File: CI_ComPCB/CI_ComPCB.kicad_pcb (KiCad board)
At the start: 2 copper layers, 121.9 x 86.4 mm, 73 parts, among them IC301 TPS63020DSJR, IC401 TPS54331DR, J101 Conn_01x01_Male, J301 Connector_Conn_01x01_Male, J302 Connector_Conn_01x01_Male, J303 Connector_Conn_01x01_Male, J401 Connector_Conn_01x01_Male, J402 Conn_01x02_Male, J403 Conn_01x01_Male, J501 RJ45_LED_Shielded, J502 RJ45_LED_Shielded, J601 Conn_01x02_Male, J602 Conn_01x02_Male, J603 Conn_01x03_Male, J604 Conn_01x03_Male, J605 Conn_01x02_Male, K601 SRD-05VDC-SL-C, K602 SRD-05VDC-SL-C, Q201 Transistor_FET_IRF9540N, Q601 2N3904, Q602 2N3904, U101 ESP32s

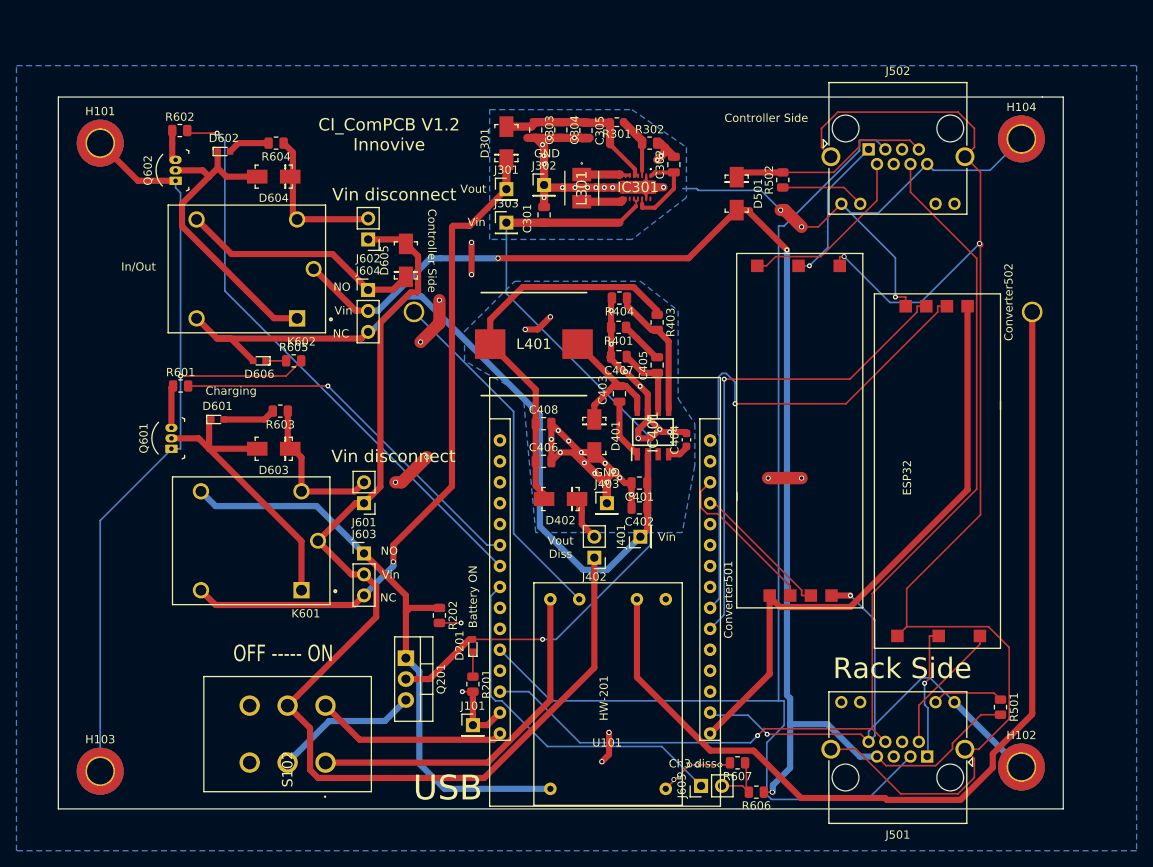
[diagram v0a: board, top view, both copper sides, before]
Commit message: Production1
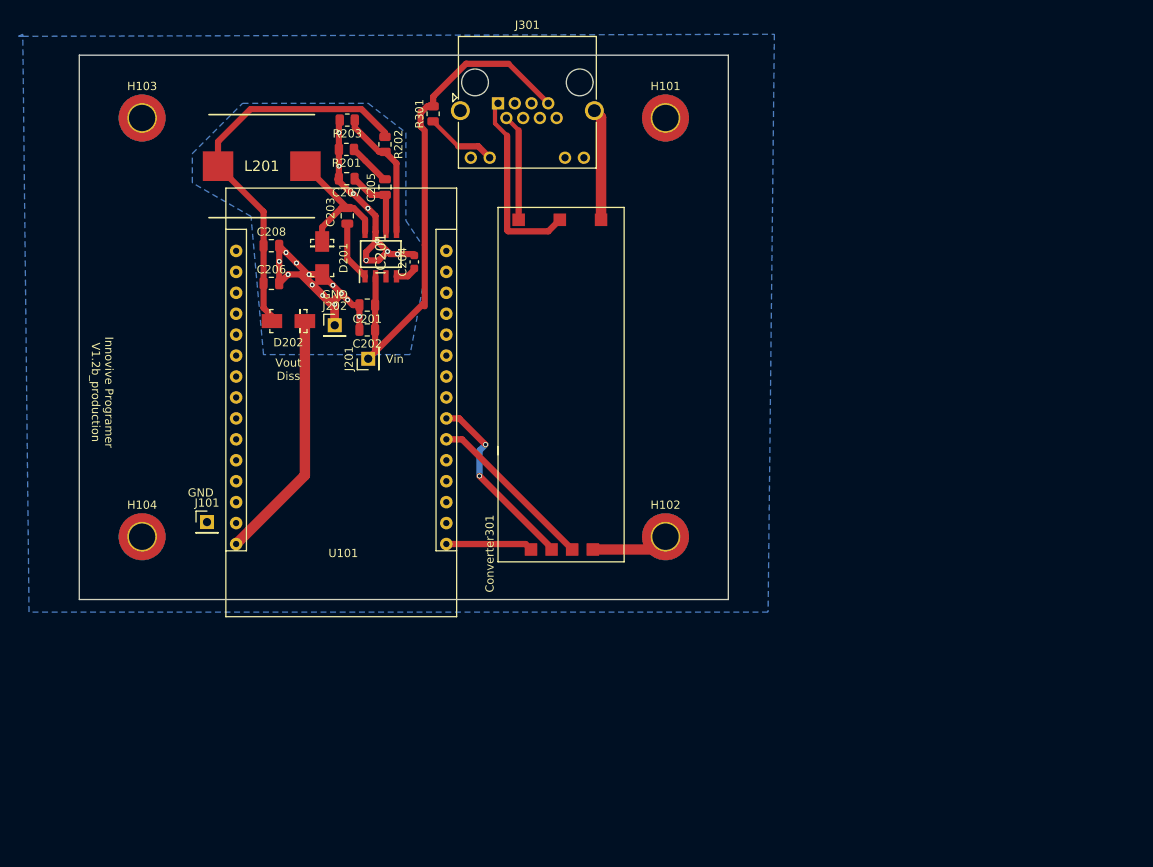
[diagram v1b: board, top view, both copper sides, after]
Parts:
- removed C301: 22uF, Capacitor_SMD:C_0805_2012Metric
- removed C302: 100nF, Capacitor_SMD:C_0805_2012Metric
- removed C303, C304, C305: 10uf, Capacitor_SMD:C_0805_2012Metric
- removed Converter501, Converter502: TxRx-RS485, CI_ComPCB:TXRX-AB
- removed the D201 at (145.8, 138.1)
- removed D301, D501, D605: SS34, digikey-footprints:DO-214AC
- removed D601, D602, D606: LTST-C190GKT, digikey-footprints:LED_0603
- removed D603, D604: 1N4007, digikey-footprints:DO-214AC
- removed HW-201: Charger-New_Library-RackComm-rescue-RackComm-rescue, CI_ComPCB:Charger
- removed Holder201: Battery-New_Library-RackComm-rescue, CI_ComPCB:Battery
- removed IC301: TPS63020DSJR, SamacSys_Parts:TPS63020DSJR
- removed J302, J303: Connector_Conn_01x01_Male, Connector_PinHeader_2.54mm:PinHeader_1x01_P2.54mm_Vertical
- removed J402, J601, J602, J605: Conn_01x02_Male, Connector_PinHeader_2.54mm:PinHeader_1x02_P2.54mm_Vertical
- removed J501, J502: RJ45_LED_Shielded, Connector_RJ:RJ45_Amphenol_RJHSE538X
- removed J603, J604: Conn_01x03_Male, Connector_PinHeader_2.54mm:PinHeader_1x03_P2.54mm_Vertical
- removed K601, K602: SRD-05VDC-SL-C, SRD-05VDC-SL-C:RELAY_SRD-05VDC-SL-C
- removed L301: SPM4012T-1R0M-LR, SamacSys_Parts:SPM4010-4020
- removed Q201: Transistor_FET_IRF9540N, Package_TO_SOT_THT:TO-220-3_Vertical
- removed Q601, Q602: 2N3904, digikey-footprints:TO-92-3
- removed the R201 at (145.8, 142.8)
- removed the R202 at (141.7, 134.4)
- removed R302: 130k, Resistor_SMD:R_0805_2012Metric
- removed R501, R502, R605: 680, Resistor_SMD:R_0805_2012Metric
- removed R601, R602: 5.6k, Resistor_SMD:R_0805_2012Metric
- removed R603, R604: 1k, Resistor_SMD:R_0805_2012Metric
- removed R606: 11k, Resistor_SMD:R_0805_2012Metric
- removed R607: 29k, Resistor_SMD:R_0805_2012Metric
- removed S102: L202021MA04QE, SamacSys_Parts:L202021MA04QE
- added Converter301: TxRx-RS485, CI_ComPCB:TXRX-AB, F.Cu at (148.8, 127.9)
- J301: value Connector_Conn_01x01_Male -> RJ45_LED_Shielded; footprint Connector_PinHeader_2.54mm:PinHeader_1x01_P2.54mm_Vertical -> Connector_RJ:RJ45_Amphenol_RJHSE538X
- R301: value 1.27M -> 680; footprint Resistor_SMD:R_0603_1608Metric -> Resistor_SMD:R_0805_2012Metric
- moved H104 117.1 mm to (105.6, 124.9)
- moved H103 79.4 mm to (105.6, 74.1)
- moved H101 68.6 mm to (169.1, 74.1)
- moved H102 51.4 mm to (169.1, 124.9)
- moved J101 40.6 mm to (113.5, 123.1)
- moved C204 39.5 mm to (138.7, 91.6)
- moved C206 39.5 mm to (121.3, 94.2)
- moved C208 39.5 mm to (121.3, 89.6)
- moved IC201 39.5 mm to (134.6, 90.6)
- moved J201 39.5 mm to (133.1, 103.3)
- moved R201 39.5 mm to (130.4, 77.9)
- moved D201 39.5 mm to (127.5, 91.1)
- moved L201 39.5 mm to (120.2, 79.9)
- moved C202 39.5 mm to (133.0, 99.8)
- moved C203 39.5 mm to (130.5, 86.0)
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- renumbered C401 to C201, C402 to C202, C403 to C203, C404 to C204, C405 to C205, C406 to C206, C407 to C207, C408 to C208, D401 to D201, D402 to D202, IC401 to IC201, J401 to J201, J403 to J202, L401 to L201, R401 to R201, R403 to R202, R404 to R203
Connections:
- C201 pad 1: Buck_IN -> EPower
- C202 pad 1: Buck_IN -> EPower
- D202 pad 1: Net-(D402-Pad1) -> Vin
- IC201 pad 2: Buck_IN -> EPower
- J201 pad 1: Buck_IN -> EPower
- J301 pad 1: Buck_Converter_OUT -> B1
- R301 pad 1: Net-(IC301-Pad3) -> Net-(J301-Pad10)
- R301 pad 2: Net-(C303-Pad1) -> EPower
- U101 pad D13: RX1 -> Net-(U101-PadD13)
- U101 pad D14: TX1 -> Net-(U101-PadD14)
- U101 pad D25: Ch3 -> Net-(U101-PadD25)
- U101 pad D32: Ch1 -> Net-(U101-PadD32)
- U101 pad D33: Ch2 -> Net-(U101-PadD33)
- U101 pad RX0: RX0 -> Net-(U101-PadRX0)
- U101 pad TX0: TX0 -> Net-(U101-PadTX0)
- U101 pad Vin: ESP_Power -> Vin
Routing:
- net GND: track 397.9 -> 88.7 mm, vias 58 -> 20
- net Sheild: track 168.0 -> 0.00 mm, vias 2 -> 0
- net TX1: track 145.1 -> 0.00 mm
- net Net-(HW-201-Pad2): track 139.5 -> 0.00 mm
- net RX1: track 127.9 -> 0.00 mm, vias 1 -> 0
- net Vin: track 138.5 -> 30.5 mm
- net Charger_OUT: track 103.6 -> 0.00 mm, vias 1 -> 0
- net EPower: track 165.3 -> 63.6 mm, vias 3 -> 0
- net Buck_IN: track 96.2 -> 0.00 mm
- net Buck_Converter_OUT: track 82.2 -> 0.00 mm, vias 1 -> 0
- net Charger_IN: track 72.6 -> 0.00 mm
- net Ch2: track 70.5 -> 0.00 mm, vias 1 -> 0
- net 3.3V: track 72.6 -> 10.5 mm
- net Ch1: track 45.8 -> 0.00 mm, vias 1 -> 0
- net Ch3: track 43.7 -> 0.00 mm
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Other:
- board size 121.9 x 86.4 mm -> 78.7 x 66 mm
- board text added: "Innovive Programer V1.2b_production"
- board text removed: "Battery ON"
- board text removed: "CI_ComPCB V1.2 Innovive"
- board text removed: "Ch3 diss"
- board text removed: "Charging"
- board text removed: "Controller Side"
- board text removed: "ESP32"
- board text removed: "In/Out"
- board text removed: "NC"
- board text removed: "NO"
- board text removed: "OFF ----- ON"
- board text removed: "Rack Side"
- board text removed: "USB"
- board text removed: "Vin disconnect"
- board text removed: "Vout"

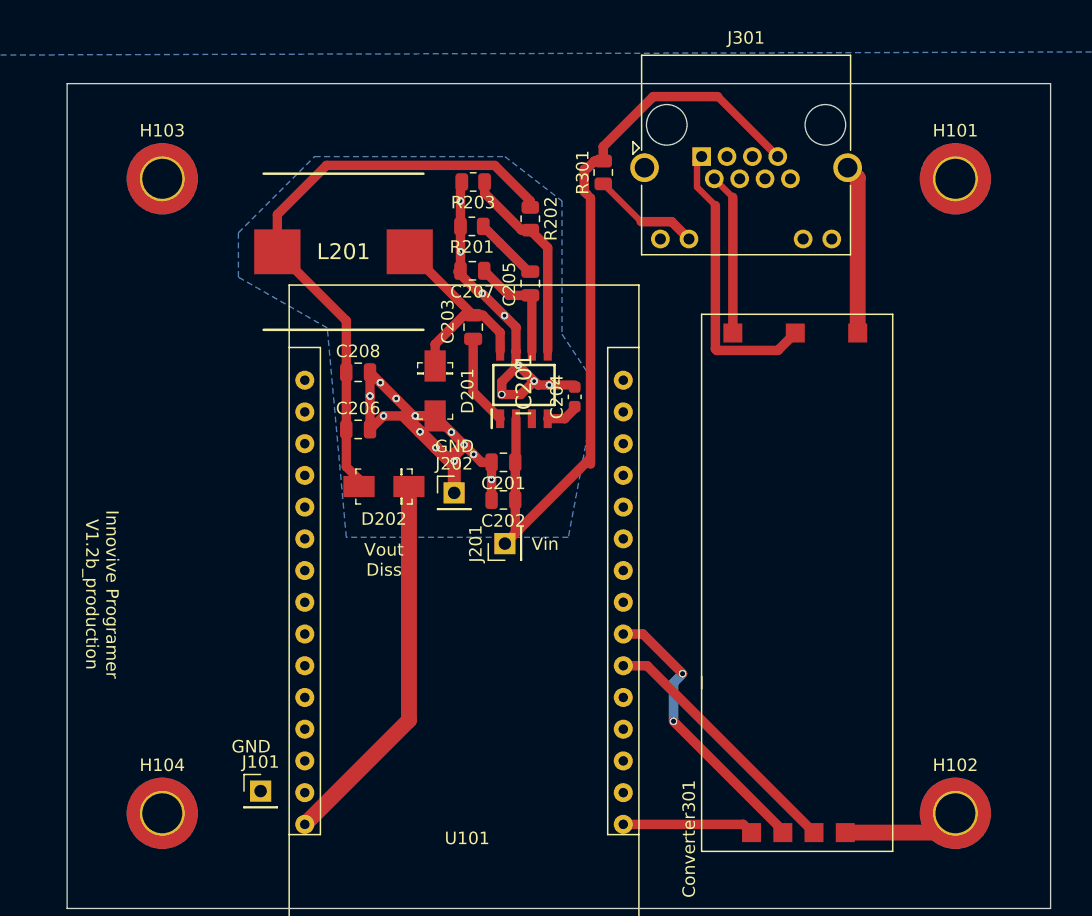
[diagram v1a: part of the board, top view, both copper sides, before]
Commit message: print
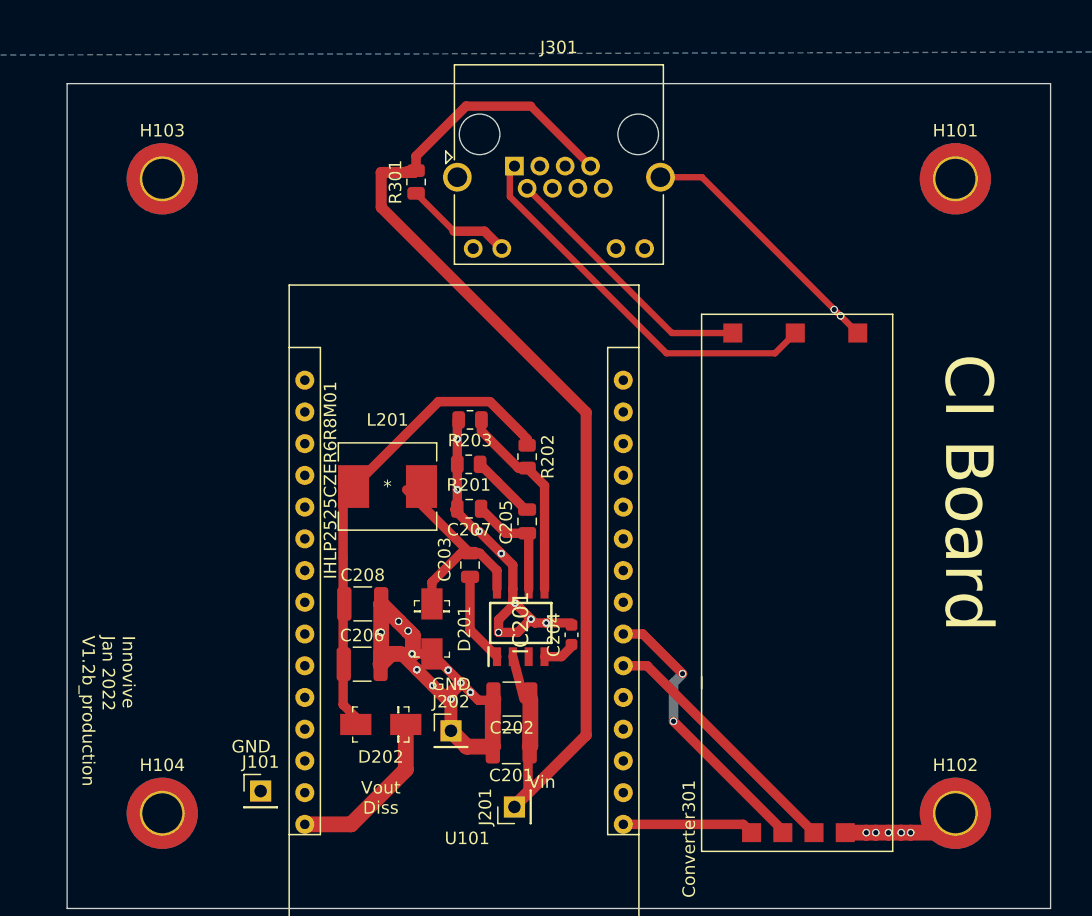
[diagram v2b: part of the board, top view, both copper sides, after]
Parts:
- C201, C202: value 10uF -> 22uf; footprint Capacitor_SMD:C_0805_2012Metric -> Capacitor_SMD:C_1210_3225Metric
- C206, C208: footprint Capacitor_SMD:C_0805_2012Metric -> Capacitor_SMD:C_1210_3225Metric
- L201: value RLF12560T-7R8N8R2 -> IHLP2525CZER6R8M01; footprint SamacSys_Parts:INDPM128125X600N -> IND:IHLP2525CZER6R8M01
- moved C201 22.8 mm to (133.6, 119.6)
- moved J201 21.1 mm to (133.8, 124.4)
- moved L201 19.1 mm to (123.7, 98.7), turned to 0 degrees
- moved C203 19.1 mm to (130.3, 105.0)
- moved C207 19.1 mm to (130.2, 100.5)
- moved J202 19.1 mm to (128.8, 118.3)
- moved C204 19.1 mm to (138.4, 110.6)
- moved C205 19.1 mm to (134.8, 101.5)
- moved D201 19.1 mm to (127.2, 110.1)
- moved D202 19.1 mm to (123.1, 117.8)
- moved IC201 19.1 mm to (134.3, 109.7)
- moved R201 19.1 mm to (130.2, 97.0)
- moved R202 19.1 mm to (134.8, 96.3)
- moved R203 19.1 mm to (130.3, 93.4)
- moved C206 18.8 mm to (121.6, 113.0)
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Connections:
- L201 pad 1: Net-(C203-Pad1) -> Net-(C206-Pad1)
- L201 pad 2: Net-(C206-Pad1) -> Net-(C203-Pad1)
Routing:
- net EPower: track 63.6 -> 93.5 mm
- net Vin: track 30.5 -> 13.5 mm
- net GND: track 88.7 -> 99.3 mm, vias 20 -> 25
- net A1: track 13.0 -> 21.3 mm
- net B1: track 23.2 -> 31.3 mm
- net Net-(C206-Pad1): track 48.9 -> 41.4 mm
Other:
- board text added: "CI Board"
- board text added: "Innovive Jan 2022 V1.2b_production"
- board text removed: "Innovive Programer V1.2b_production"
